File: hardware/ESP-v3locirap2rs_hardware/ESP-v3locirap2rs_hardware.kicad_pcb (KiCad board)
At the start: 2 copper layers, 53.5 x 77 mm, 3 parts, among them U1 ESP32-DEVKITC-32D

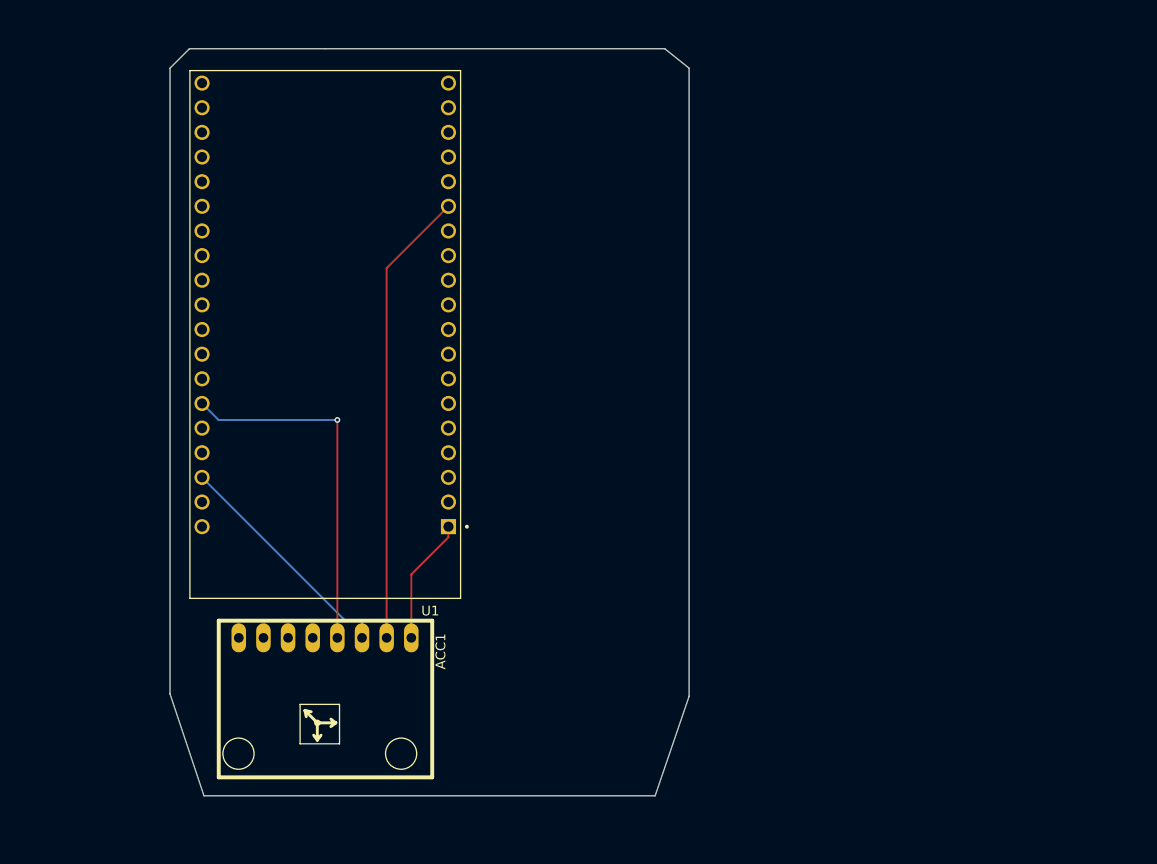
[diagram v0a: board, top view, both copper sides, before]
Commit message: PCB completed
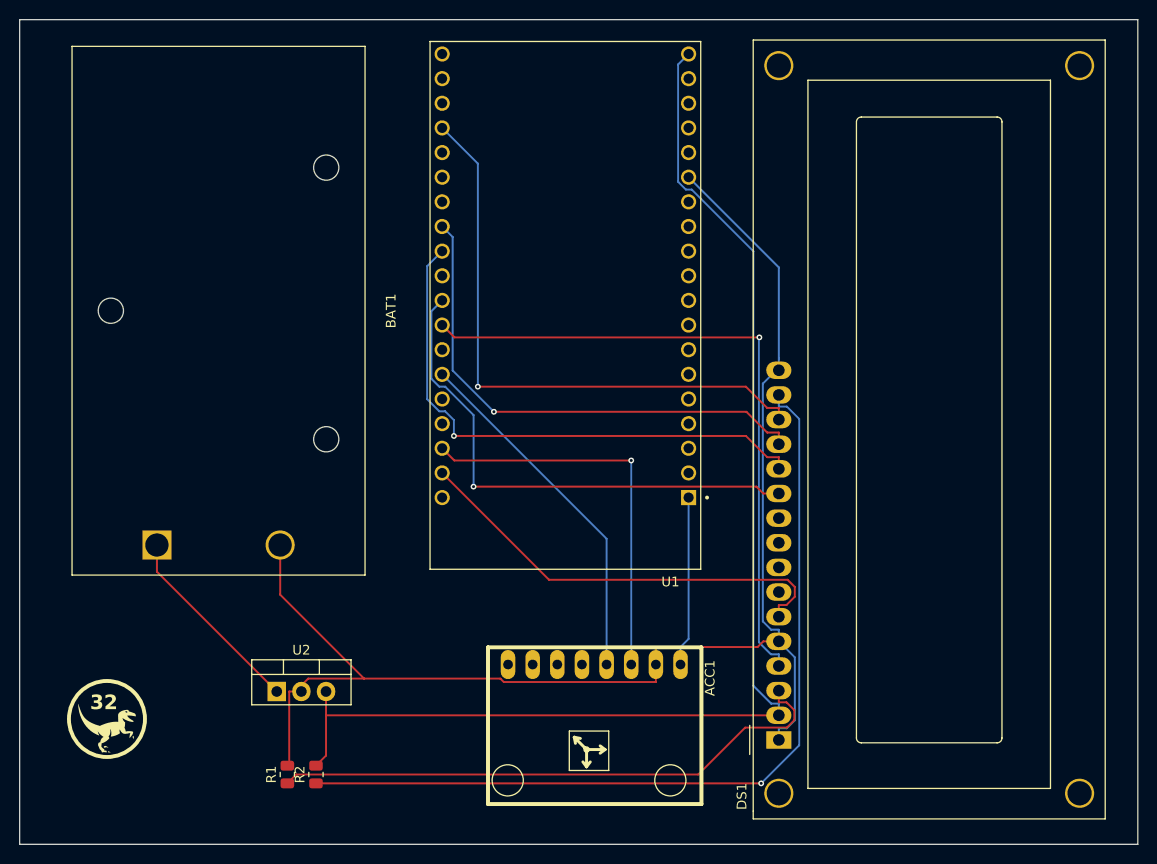
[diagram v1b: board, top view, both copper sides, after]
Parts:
- added BAT1: BC9VPC, Battery:BatteryHolder_Eagle_12BH611-GR, F.Cu at (95.2, 103.7)
- added DS1: WC1602A, Display:WC1602A, F.Cu at (159.2, 123.7)
- added R1: 1k, Resistor_SMD:R_0805_2012Metric, F.Cu at (108.6, 127.3)
- added R2: 1.2k, Resistor_SMD:R_0805_2012Metric, F.Cu at (111.5, 127.3)
- added U2: L7805CV, Package_TO_SOT_THT:TO-220-3_Vertical, F.Cu at (107.5, 118.8)
- G***: moved to F.Cu
- moved ACC1 27.9 mm to (129.3, 114.2)
- moved U1 24.9 mm to (137.2, 79.0)
- moved G*** 22.5 mm to (90.0, 122.5), turned to 0 degrees
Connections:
- U1 pad J2-19: unconnected-(U1-EXT_5V-PadJ2-19) -> /ESP32/5V
- U1 pad J3-11: unconnected-(U1-IO17-PadJ3-11) -> /ESP32/Pin 17
- U1 pad J3-12: unconnected-(U1-IO16-PadJ3-12) -> /ESP32/Pin 16
- U1 pad J3-16: unconnected-(U1-IO15-PadJ3-16) -> /ESP32/Pin 15
- U1 pad J3-2: unconnected-(U1-IO23-PadJ3-2) -> /ESP32/Pin 23
- U1 pad J3-8: unconnected-(U1-IO19-PadJ3-8) -> /ESP32/Pin 19
- U1 pad J3-9: unconnected-(U1-IO18-PadJ3-9) -> /ESP32/Pin 18
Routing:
- net /ESP32/5V: track 0.00 -> 128.5 mm
- net GND: track 47.1 -> 146.5 mm
- net Net-(DS1-LED(+)): track 0.00 -> 88.9 mm, vias 0 -> 1
- net /ESP32/Pin 19: track 0.00 -> 68.4 mm, vias 0 -> 1
- net /ESP32/Pin 15: track 0.00 -> 61.3 mm, vias 0 -> 1
- net Net-(DS1-VO): track 0.00 -> 59.1 mm
- net /ESP32/Pin 17: track 0.00 -> 56.8 mm, vias 0 -> 1
- net /ESP32/Pin 18: track 0.00 -> 53.6 mm, vias 0 -> 1
- net /ESP32/Pin 16: track 0.00 -> 52.8 mm, vias 0 -> 1
- net /ESP32/Pin 23: track 0.00 -> 45.4 mm
- net Net-(U2-IN): track 0.00 -> 20.2 mm
- net /ESP32/SCL: track 24.4 -> 41.0 mm, vias 0 -> 1
- net /ESP32/3.3V: track 13.0 -> 17.6 mm
- net unconnected-(ACC1-PadXCL): track 0.64 -> 0.00 mm
- net /ESP32/SDA: track 37.1 -> 36.9 mm, vias 1 -> 0
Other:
- board size 53.5 x 77 mm -> 115.2 x 85 mm

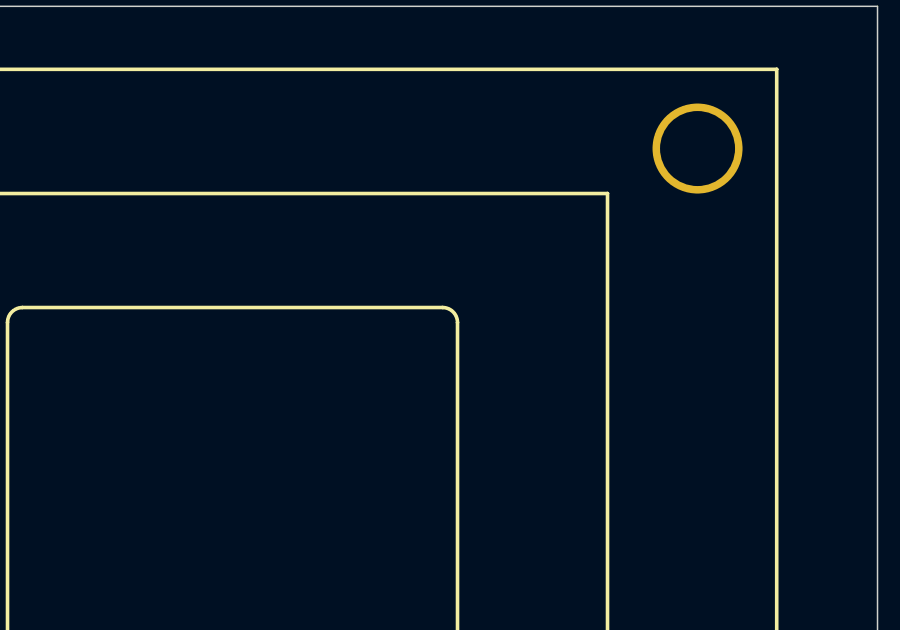
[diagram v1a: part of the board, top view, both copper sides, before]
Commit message: pcb & schematic updates
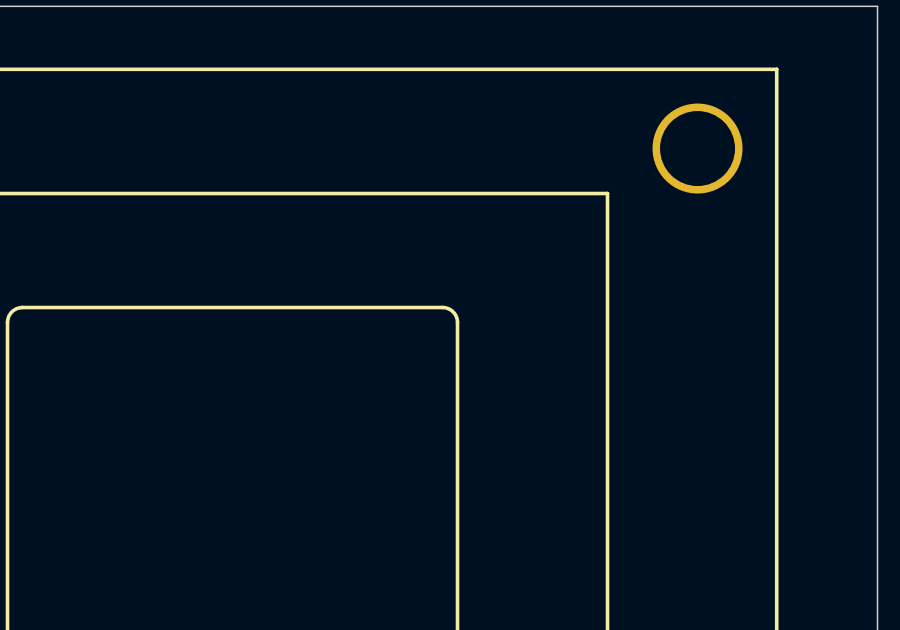
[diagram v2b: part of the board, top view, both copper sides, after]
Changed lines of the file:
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@@
 		(fp_arc
 			(start 64.20104 22.49932)
-			(mid 64.054473 22.853115)
+			(mid 64.054479 22.85315)
 			(end 63.70066 22.9997)
 			(stroke
